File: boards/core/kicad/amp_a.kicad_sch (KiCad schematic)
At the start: 44 parts, among them J6 SPK A L, J7 SPK A R, U15 TPA3220

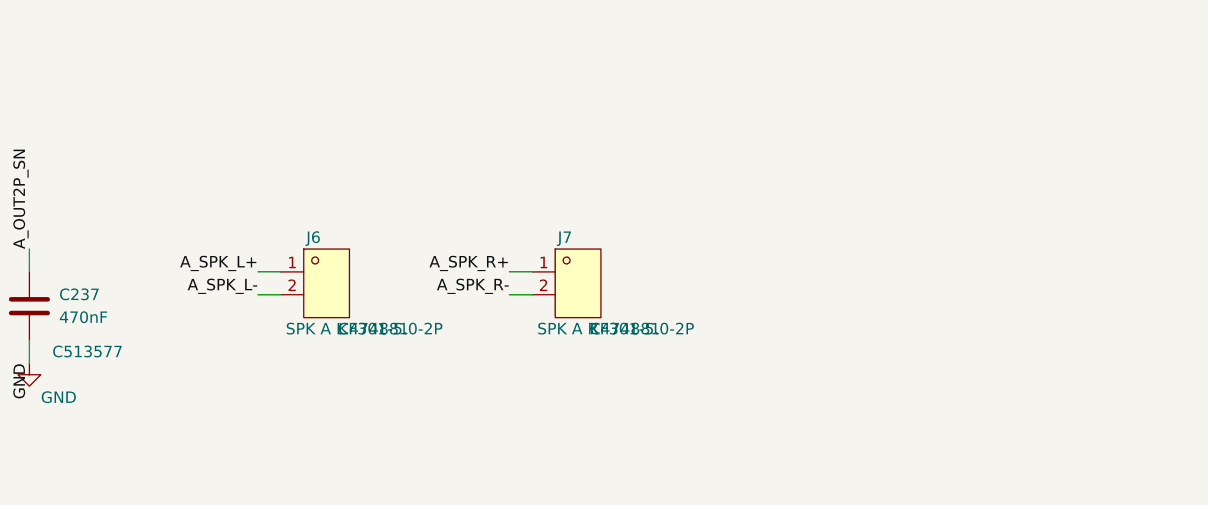
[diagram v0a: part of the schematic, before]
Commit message: WIP core banana: schematic, parts, stage-1 ECO, sockets placed
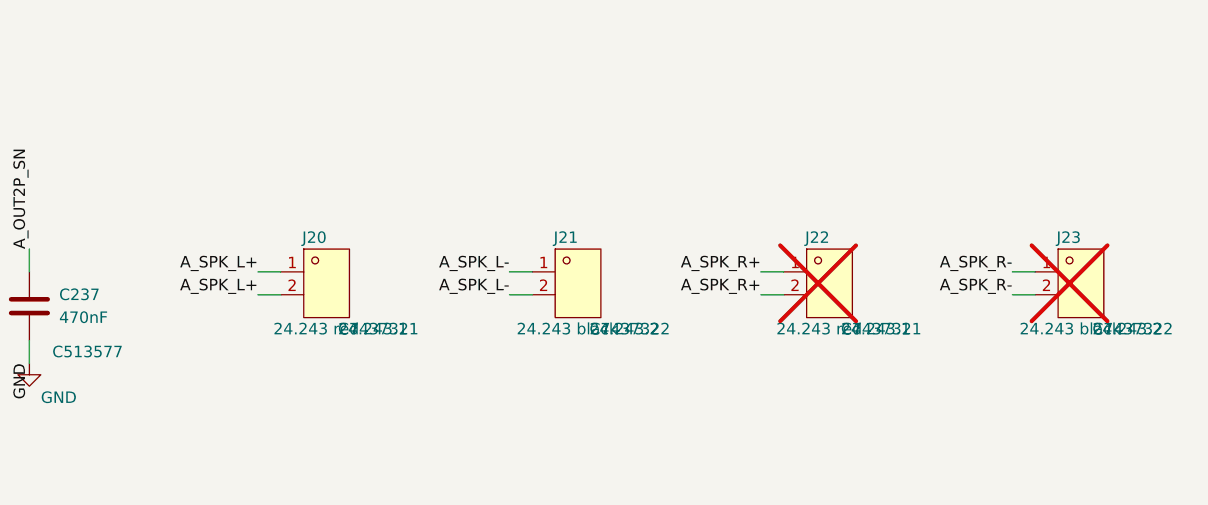
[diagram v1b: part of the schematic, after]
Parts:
- removed J6: SPK A L, aiee:CONN-TH_P5.00_KF301-5.0-2P, symbol aiee:KF301-5.0-2P
- removed J7: SPK A R, aiee:CONN-TH_P5.00_KF301-5.0-2P, symbol aiee:KF301-5.0-2P
- added J20, J22: 24.243 red, aiee:CONN-TH_24.243.1_RED, symbol aiee:24.243.1
- added J21, J23: 24.243 black, aiee:CONN-TH_24.243.2, symbol aiee:24.243.2
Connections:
- net A_SPK_L+: now also J20.1, J20.2
- net A_SPK_L-: now also J21.1, J21.2
- net A_SPK_R+: now also J22.1, J22.2
- net A_SPK_R-: now also J23.1, J23.2
